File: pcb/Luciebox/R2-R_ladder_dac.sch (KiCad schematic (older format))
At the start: 25 parts, among them T2 terminal_8x1

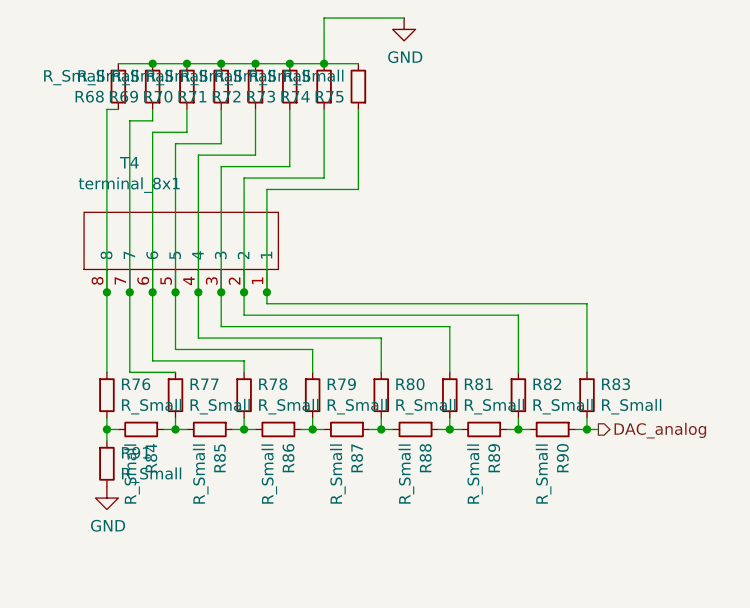
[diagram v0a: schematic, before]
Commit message: pcb progress dedicated R-2R ladder'
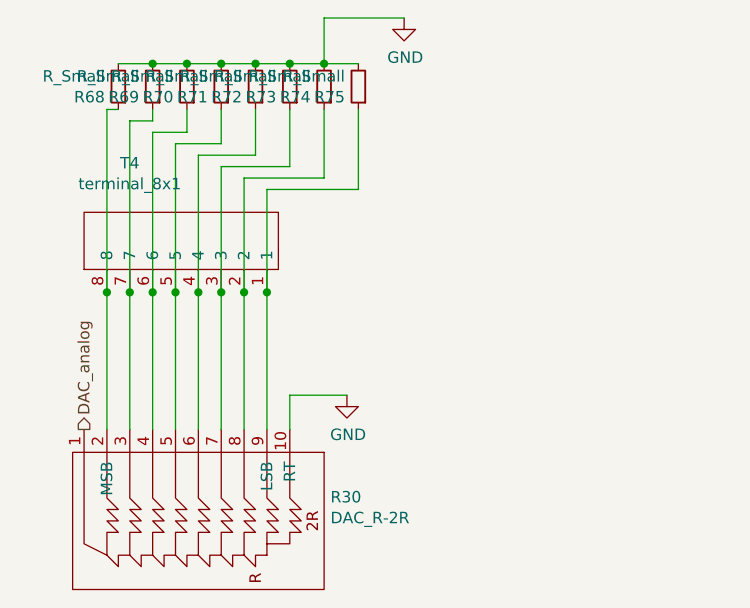
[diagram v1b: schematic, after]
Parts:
- removed R28, R29, R30, R31, R32, R33, R34, R35, R36, R37, R38, R39, R40, R41, R42, R43: R_Small, Luciebox:1206, symbol Device:R_Small
- added R28: DAC_R-2R, Luciebox:SIP-10, symbol Luciebox_components:DAC_R-2R
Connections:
- net DAC_analog: now also R28.1
- net GND: now also R28.10 (RT)
- net at R20.1, T2.8: now also R28.2 (MSB)
- net at R27.1, T2.1: now also R28.9 (LSB)
- net at R26.1, T2.2: now also R28.8
- net at R25.1, T2.3: now also R28.7
- net at R24.1, T2.4: now also R28.6
- net at R23.1, T2.5: now also R28.5
- net at R22.1, T2.6: now also R28.4
- net at R21.1, T2.7: now also R28.3
